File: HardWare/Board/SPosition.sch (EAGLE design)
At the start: 64 parts

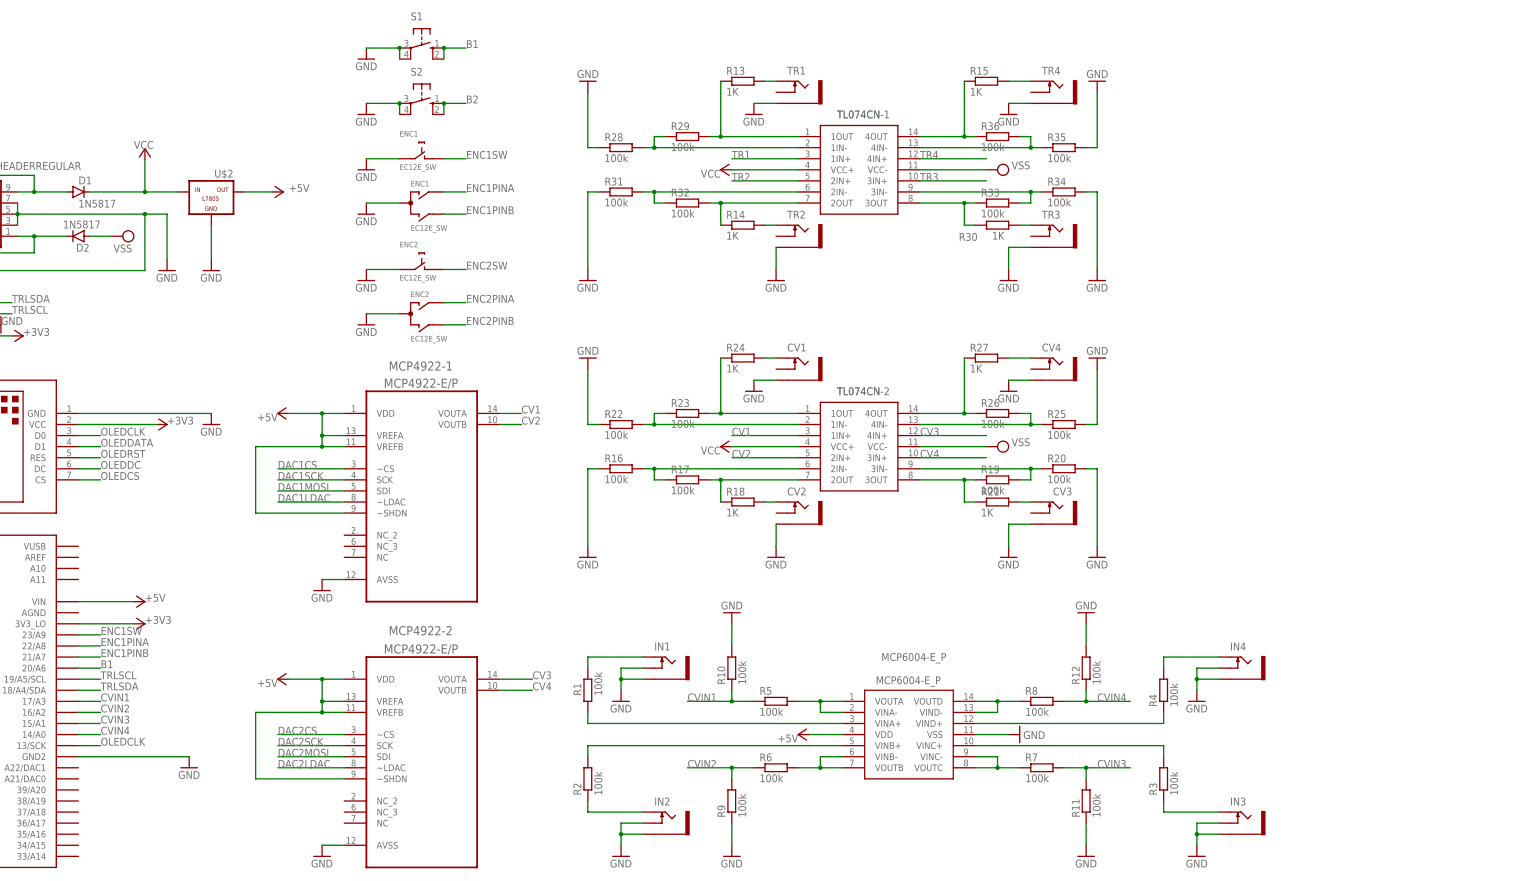
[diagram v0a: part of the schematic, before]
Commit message: board and schem revisions
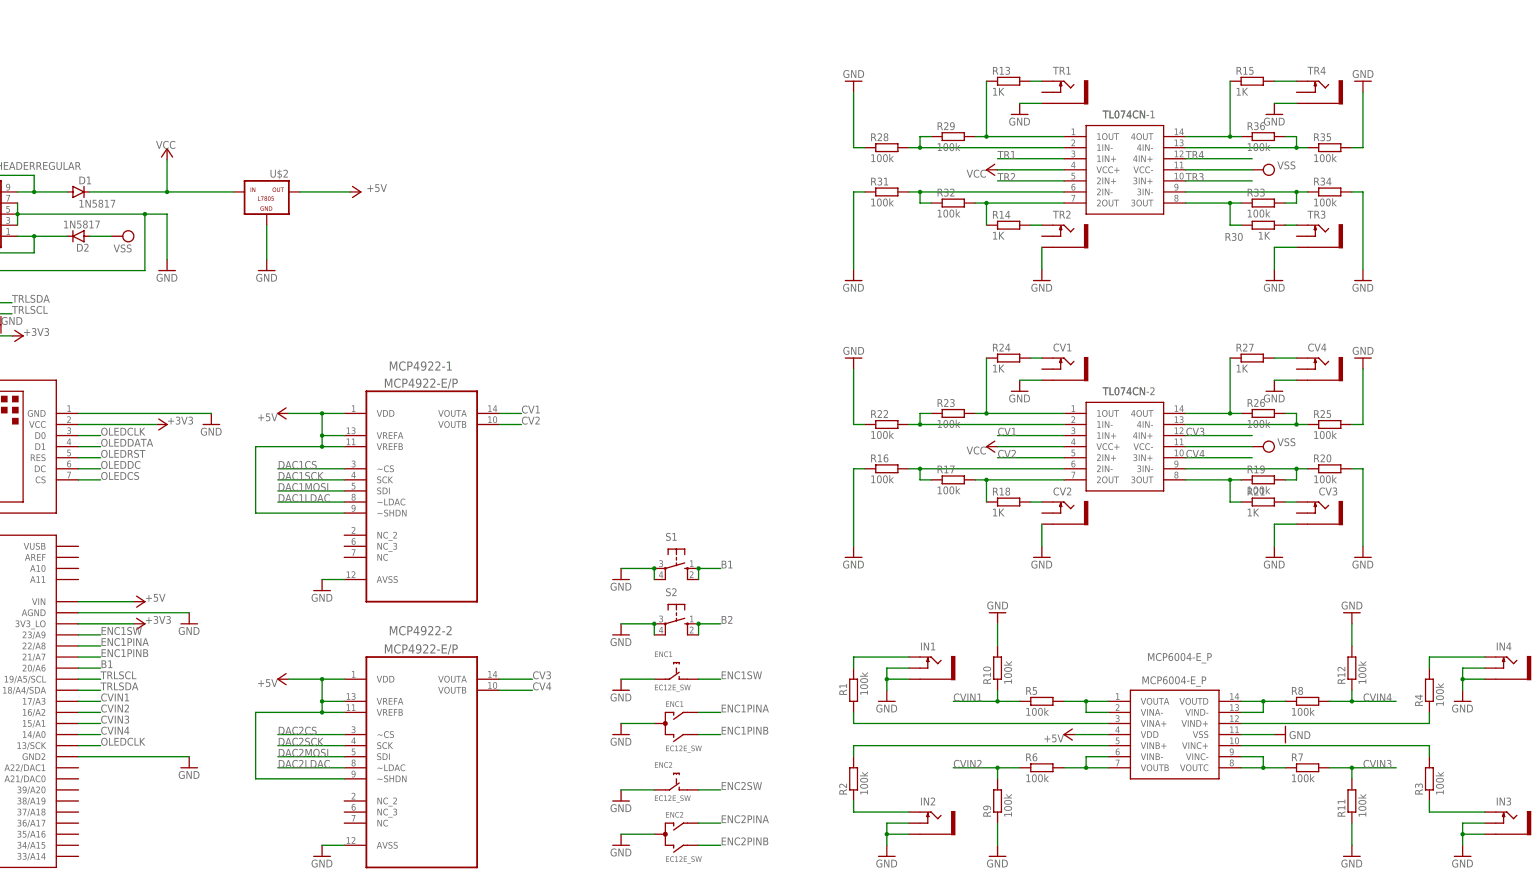
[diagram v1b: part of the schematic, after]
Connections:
- net GND: now also U$1.AGND
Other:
- moved on the sheet: CV1, CV2, CV3, CV4, ENC1, ENC2, IN1, IN2, IN3, IN4, MCP6004-E_P, R1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

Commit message: schematic and pcb rev4
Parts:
- added C1-10UF, C2-10UF: 10uF, rcl:C-EUC0805
- added C3-100N, C4-100N, C5-100N, C6-100N, C7-100N, C8-100N: 100n, rcl:C-EUC0805
- R1, R10, R11, R12, R13, R14, R15, R16, R17, R18, R19, R2, R20, R21, R22, R23, R24, R25, R26, R27, R28, R29, R3, R30, R31, R32, R33, R34, R35, R36, R4, R5, R6, R7, R8, R9: device Clean-Kong:R-EU_R0805 -> rcl:R-EU_R0805
- S1, S2: value (none) -> SW9mm
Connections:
- net +5V: now also C2-10UF.1, C3-100N.1, C4-100N.1
- net GND: now also C1-10UF.2, C2-10UF.2, C3-100N.2, C4-100N.2, C5-100N.2, C6-100N.2, C7-100N.2, C8-100N.2
- net VCC: now also C1-10UF.1, C5-100N.1, C6-100N.1
- net VSS: now also C7-100N.1, C8-100N.1
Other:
- moved on the sheet: CV1, CV2, CV3, CV4, D1, D2, ENC1, ENC2, IN1, IN2, IN3, IN4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
